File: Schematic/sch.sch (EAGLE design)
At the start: 56 parts, among them IC1 MCP23S17SP, IC2 MCP23S17SP, IC3 MCP23S17SP, IC4 74LS165N, J1 AVR_SPI_PROG2PTH, U1 ATMEGA328P-PU

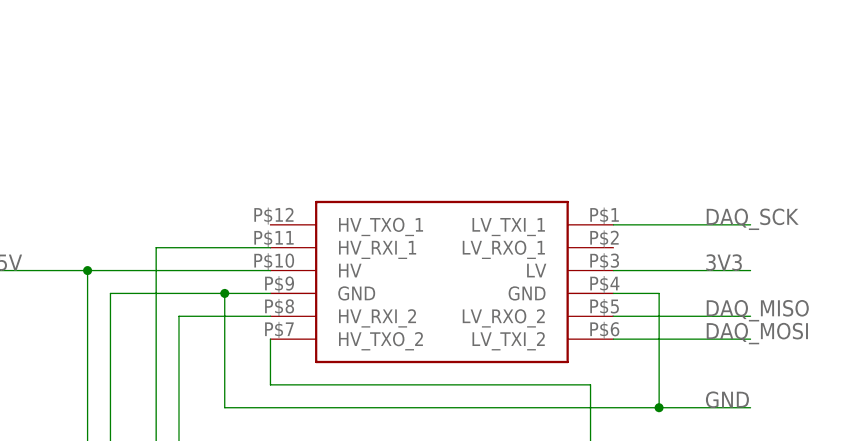
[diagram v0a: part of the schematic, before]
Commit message: Need paid version
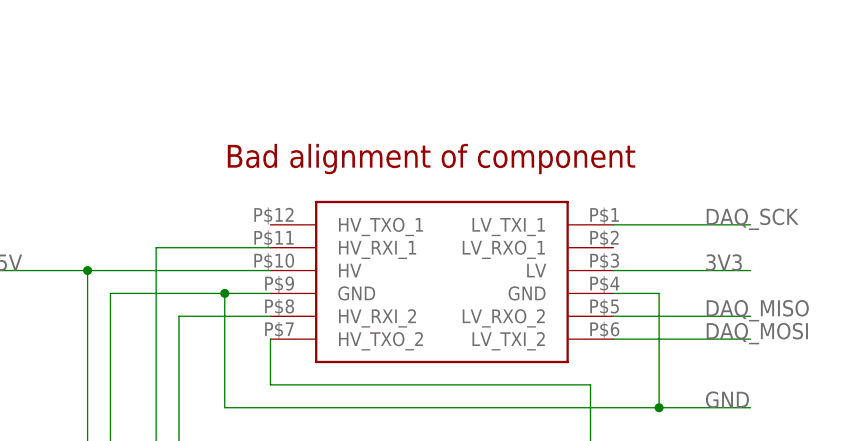
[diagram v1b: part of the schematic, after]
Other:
- note added: "Bad alignment of component"
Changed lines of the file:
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@@
 <sheet>
 <plain>
+<text x="231.14" y="312.42" size="2.54" layer="94" align="center">Bad alignment of component</text>
 </plain>
 <instances>

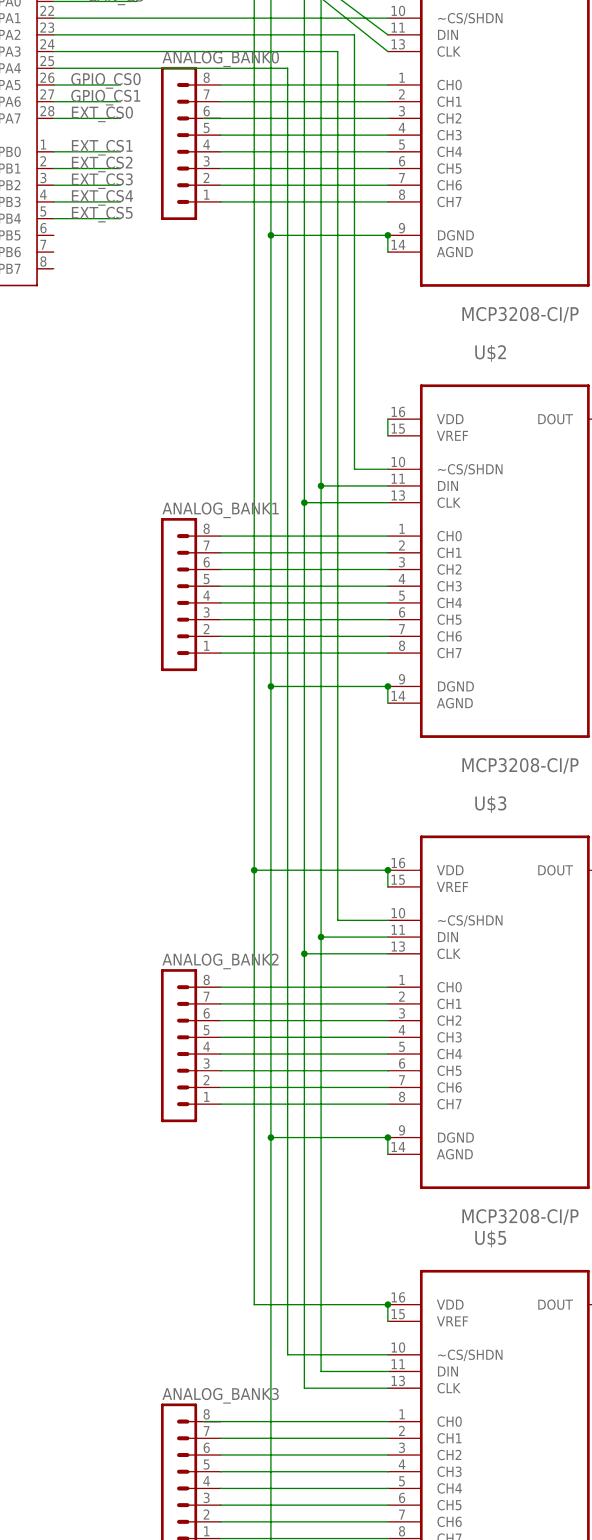
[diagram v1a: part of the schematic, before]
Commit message: Errors to be fixed
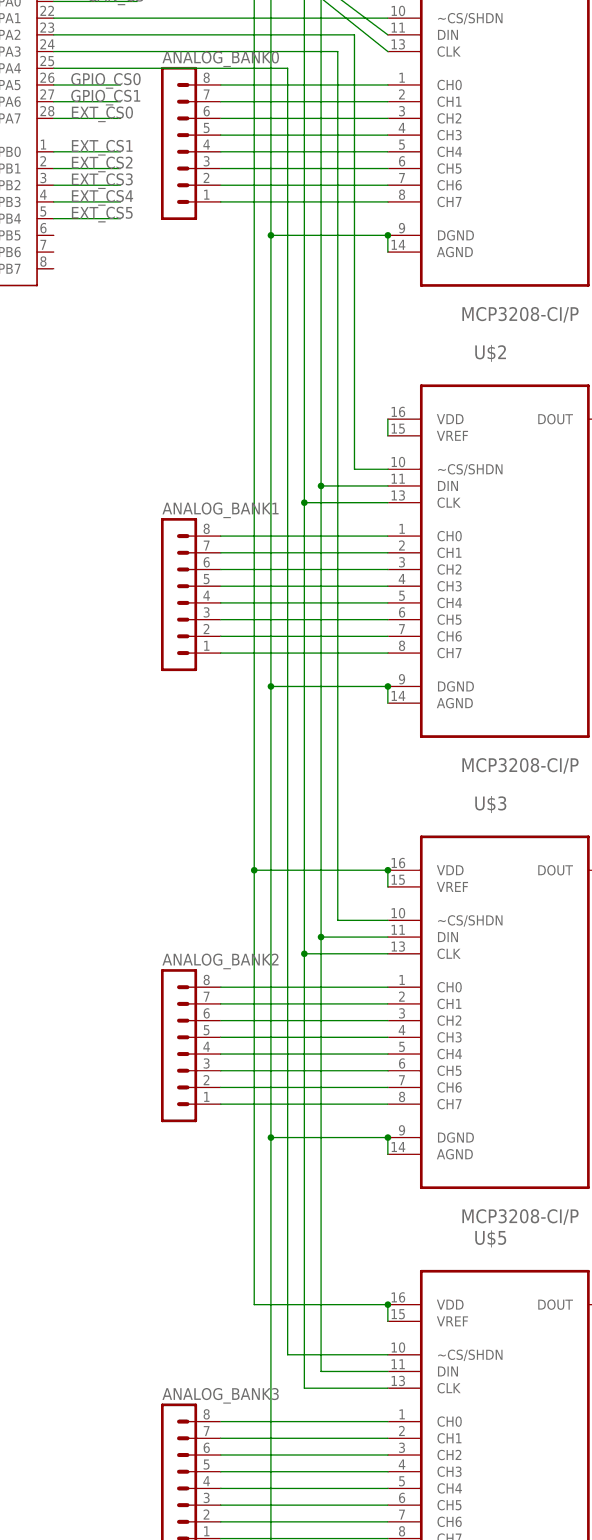
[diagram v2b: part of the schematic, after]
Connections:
- removed net N$59: U$5.CH0
- removed net N$88: U$1.CH2
- new net N$18: ANALOG_BANK3.8, U$5.CH0
- new net N$19: ANALOG_BANK0.6, U$1.CH2
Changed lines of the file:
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@@
-</segment>
-</net>
-<net name="N$59" class="0">
-<segment>
-<pinref part="U$5" gate="A" pin="CH0"/>
-<wire x1="213.36" y1="43.18" x2="185.42" y2="43.18" width="0.1524" layer="91"/>
 </segment>
 </net>
@@
 </segment>
 </net>
-<net name="N$88" class="0">
-<segment>
-<pinref part="U$1" gate="A" pin="CH2"/>
-<wire x1="213.36" y1="241.3" x2="185.42" y2="241.3" width="0.1524" layer="91"/>
-</segment>
-</net>
 <net name="N$89" class="0">
 <segment>
@@
 </segment>
 </net>
+<net name="N$18" class="0">
+<segment>
+<pinref part="ANALOG_BANK3" gate="1" pin="8"/>
+<pinref part="U$5" gate="A" pin="CH0"/>
+<wire x1="187.96" y1="43.18" x2="213.36" y2="43.18" width="0.1524" layer="91"/>
+</segment>
+</net>
+<net name="N$19" class="0">
+<segment>
+<pinref part="ANALOG_BANK0" gate="1" pin="6"/>
+<pinref part="U$1" gate="A" pin="CH2"/>
+<wire x1="187.96" y1="241.3" x2="213.36" y2="241.3" width="0.1524" layer="91"/>
+</segment>
+</net>
